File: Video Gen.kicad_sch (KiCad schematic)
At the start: 35 parts, among them J18 Aux Video, K14 RCA Connector, Q3 2N3904

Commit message: more tracing
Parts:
- K14: DigiKey (none) -> PJRAN1X1U03X-ND
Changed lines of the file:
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@@
       (effects (font (size 1.27 1.27)) hide)
     )
-    (pin "8")
-    (pin "9")
     (pin "1")
     (pin "10")
@@
     (pin "6")
     (pin "7")
+    (pin "8")
+    (pin "9")
     (instances
       (project "AppleII"
@@
     (pin "1")
     (pin "2")
-    (pin "4")
-    (pin "7")
-    (pin "8")
-    (pin "3")
-    (pin "6")
+    (pin "3")
+    (pin "4")
+    (pin "6")
+    (pin "7")
+    (pin "8")
     (instances
       (project "AppleII"
@@
       (effects (font (size 1.27 1.27)) hide)
     )
+    (pin "1")
+    (pin "2")
+    (pin "3")
+    (pin "4")
+    (pin "5")
+    (pin "6")
     (pin "8")
     (pin "9")
+    (pin "10")
     (pin "11")
-    (pin "7")
-    (pin "6")
-    (pin "10")
+    (pin "12")
+    (pin "13")
     (pin "14")
-    (pin "13")
-    (pin "1")
-    (pin "4")
-    (pin "5")
-    (pin "2")
-    (pin "3")
-    (pin "12")
+    (pin "7")
     (instances
       (project "AppleII"
@@
       (effects (font (size 1.27 1.27)) hide)
     )
-    (property "Datasheet" "" (at 215.392 67.31 0)
-      (effects (font (size 1.27 1.27)) hide)
-    )
+    (property "Datasheet" "https://www.switchcraft.com/assets/1/24/pjran1x1u__x_series_cd.pdf?4664" (at 215.392 67.31 0)
+      (effects (font (size 1.27 1.27)) hide)
+    )
+    (property "DigiKey" "PJRAN1X1U03X-ND" (at 215.392 67.31 0)
+      (effects (font (size 1.27 1.27)) hide)
+    )

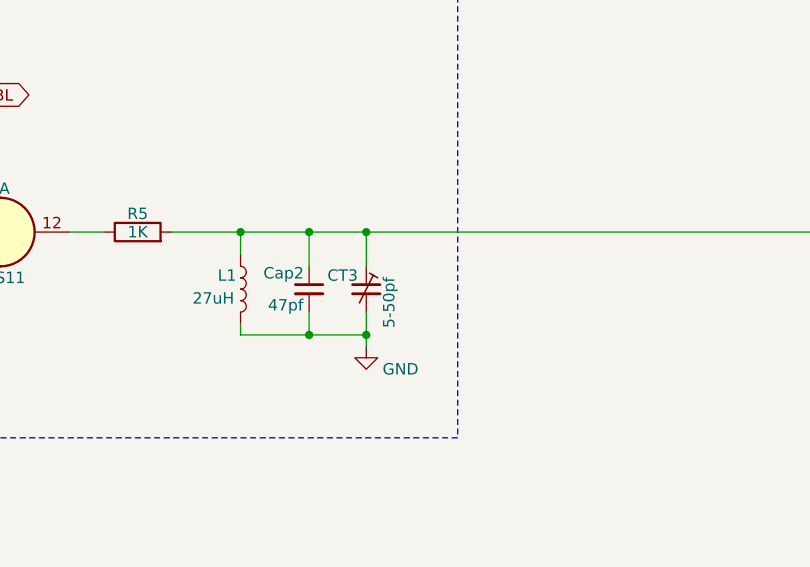
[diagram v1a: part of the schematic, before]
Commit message: more tracing
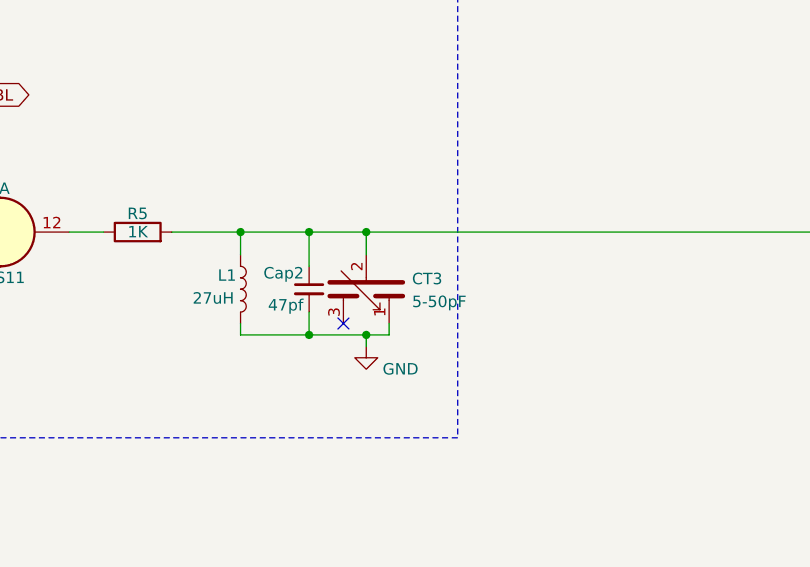
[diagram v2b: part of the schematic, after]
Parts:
- removed CT3: 5-50pf, symbol AppleII-rescue:CTRIM_Small-Device
- added CT3: 5-50pF, Apple-II:COLOUR_TRIM, symbol Device:C_Trim_Differential
- J18: footprint (none) -> Connector_PinHeader_2.54mm:PinHeader_1x04_P2.54mm_Vertical
- Q3: footprint digikey-footprints:TO-92-3 -> Package_TO_SOT_THT:TO-92
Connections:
- net GND: now also CT3.1
- net at Cap2.1, L1.1, R5.2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: now also CT3.2
- no-connect marks 7 -> 8
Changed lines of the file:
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@@
   (no_connect (at 425.45 309.88))
   (no_connect (at 425.45 304.8))
+  (no_connect (at 119.38 201.93))
   (no_connect (at 425.45 240.03))
   (no_connect (at 485.14 170.18))
@@
     (stroke (width 0) (type default))
   )
-  (wire (pts (xy 121.92 200.66) (xy 121.92 203.2))
+  (wire (pts (xy 124.46 201.93) (xy 124.46 203.2))
     (stroke (width 0) (type default))
   )
@@
     (stroke (width 0) (type default))
   )
+  (wire (pts (xy 124.46 203.2) (xy 121.92 203.2))
+    (stroke (width 0) (type default))
+  )
   (wire (pts (xy 196.85 71.12) (xy 205.74 71.12))
     (stroke (width 0) (type default))
@@
     (stroke (width 0) (type default))
   )
-  (wire (pts (xy 121.92 195.58) (xy 121.92 191.77))
+  (wire (pts (xy 121.92 194.31) (xy 121.92 191.77))
     (stroke (width 0) (type default))
   )
@@
     )
   )
-  (symbol (lib_id "AppleII-rescue:CTRIM_Small-Device") (at 121.92 198.12 0) (unit 1)
-    (in_bom yes) (on_board yes) (dnp no)
-    (property "Reference" "CT3" (at 117.602 196.596 0)
-      (effects (font (size 1.27 1.27)) (justify left))
-    )
-    (property "Value" "5-50pf" (at 124.46 202.438 90)
-      (effects (font (size 1.27 1.27)) (justify left))
-    )
-    (property "Footprint" "" (at 121.92 198.12 0)
-      (effects (font (size 1.27 1.27)) hide)
-    )
-    (property "Datasheet" "~" (at 121.92 198.12 0)
-      (effects (font (size 1.27 1.27)) hide)
-    )
-    (pin "1")
-    (pin "2")
-    (instances
-      (project "AppleII"
-        (path "/f1f08369-4db3-46f7-9b89-a5d3cfbed55a/00000000-0000-0000-0000-0000632bf564"
-          (reference "CT3") (unit 1)
-        )
-      )
-    )
-  )
   (symbol (lib_id "power:GND") (at 121.92 204.47 0) (unit 1)
     (in_bom yes) (on_board yes) (dnp no)
@@
       (effects (font (size 1.27 1.27)) (justify right))
     )
-    (property "Footprint" "" (at 172.72 59.69 0)
+    (property "Footprint" "Connector_PinHeader_2.54mm:PinHeader_1x04_P2.54mm_Vertical" (at 172.72 59.69 0)
       (effects (font (size 1.27 1.27)) hide)
     )
@@
       (effects (font (size 1.524 1.524)) (justify left))
     )
-    (property "Footprint" "digikey-footprints:TO-92-3" (at 168.91 92.71 0)
+    (property "Footprint" "Package_TO_SOT_THT:TO-92" (at 168.91 92.71 0)
       (effects (font (size 1.524 1.524)) (justify left) hide)
     )
@@
         )
       )
+    )
+  )
+  (symbol (lib_id "Device:C_Trim_Differential") (at 121.92 198.12 180) (unit 1)
+    (in_bom yes) (on_board yes) (dnp no) (fields_autoplaced)
+    (property "Reference" "CT3" (at 127 196.977 0)
+      (effects (font (size 1.27 1.27)) (justify right))
+    )
+    (property "Value" "5-50pF" (at 127 199.517 0)
+      (effects (font (size 1.27 1.27)) (justify right))
+    )
+    (property "Footprint" "Apple-II:COLOUR_TRIM" (at 121.92 198.12 0)
+      (effects (font (size 1.27 1.27)) hide)
+    )
+    (property "Datasheet" "https://www.vishay.com/docs/28528/bfc2808-10mm.pdf" (at 121.92 198.12 0)
+      (effects (font (size 1.27 1.27)) hide)
+    )
+    (property "DigiKey" "BFC280831659-ND" (at 121.92 198.12 0)
+      (effects (font (size 1.27 1.27)) hide)
+    )
+    (pin "1")
+    (pin "2")
+    (pin "3")
+    (instances
+      (project "AppleII"
+        (path "/f1f08369-4db3-46f7-9b89-a5d3cfbed55a/00000000-0000-0000-0000-0000632bf564"
+          (reference "CT3") (unit 1)
+        )
+      )

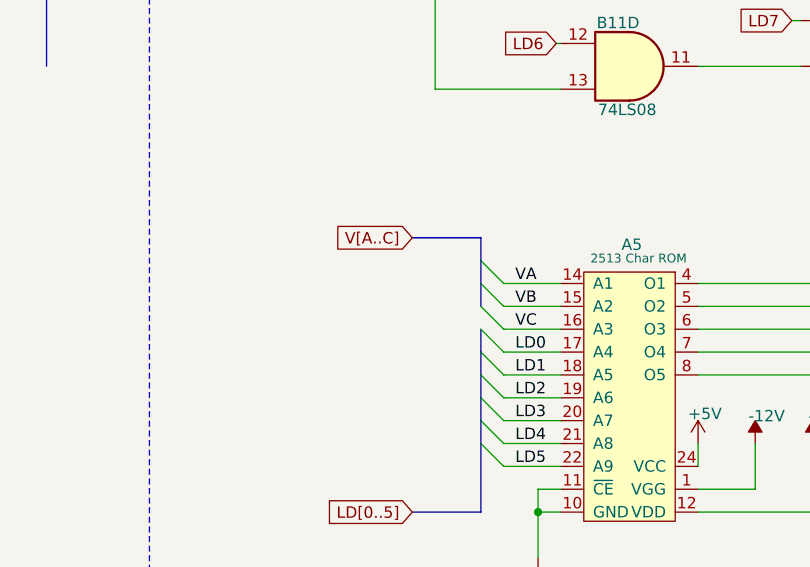
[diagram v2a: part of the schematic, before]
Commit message: more tracing
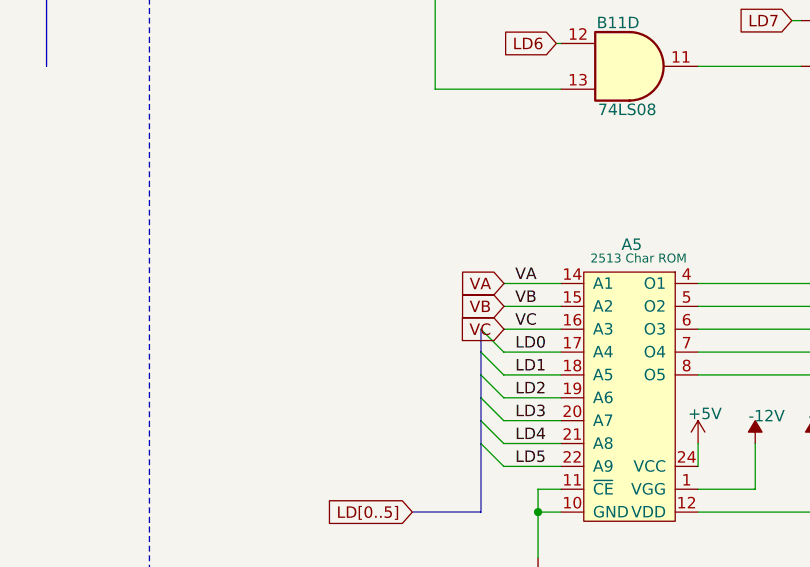
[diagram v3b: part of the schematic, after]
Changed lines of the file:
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@@
-    (stroke (width 0) (type default))
-  )
-  (bus_entry (at 302.26 135.89) (size 2.54 2.54)
     (stroke (width 0) (type default))
   )
@@
     (stroke (width 0) (type default))
   )
-  (bus_entry (at 302.26 138.43) (size 2.54 2.54)
-    (stroke (width 0) (type default))
-  )
   (bus_entry (at 395.224 242.57) (size 2.54 2.54)
     (stroke (width 0) (type default))
   )
-  (bus_entry (at 302.26 133.35) (size 2.54 2.54)
-    (stroke (width 0) (type default))
-  )
   (bus_entry (at 395.224 234.95) (size 2.54 2.54)
     (stroke (width 0) (type default))
@@
     (stroke (width 0) (type default))
   )
-  (bus (pts (xy 294.64 130.81) (xy 302.26 130.81))
-    (stroke (width 0) (type default))
-  )
   (wire (pts (xy 36.83 374.65) (xy 34.29 374.65))
     (stroke (width 0) (type default))
@@
     (stroke (width 0) (type default))
   )
-  (bus (pts (xy 302.26 133.35) (xy 302.26 130.81))
-    (stroke (width 0) (type default))
-  )
   (wire (pts (xy 153.67 95.25) (xy 157.48 95.25))
     (stroke (width 0) (type default))
@@
     (stroke (width 0) (type default))
   )
-  (bus (pts (xy 302.26 138.43) (xy 302.26 135.89))
-    (stroke (width 0) (type default))
-  )
   (wire (pts (xy 149.86 63.5) (xy 149.86 64.77))
     (stroke (width 0) (type default))
@@
   )
   (wire (pts (xy 304.8 146.05) (xy 311.15 146.05))
-    (stroke (width 0) (type default))
-  )
-  (bus (pts (xy 302.26 135.89) (xy 302.26 133.35))
     (stroke (width 0) (type default))
   )
@@
     )
   )
+  (global_label "VB" (shape input) (at 304.8227 138.43 180) (fields_autoplaced)
+    (effects (font (size 1.27 1.27)) (justify right))
+    (property "Intersheetrefs" "${INTERSHEET_REFS}" (at 300.1331 138.43 0)
+      (effects (font (size 1.27 1.27)) (justify right) hide)
+    )
+  )
   (global_label "HIRES" (shape output) (at 151.13 325.12 0)
     (effects (font (size 1.27 1.27)) (justify left))
@@
     )
   )
+  (global_label "VA" (shape input) (at 304.8227 135.89 180) (fields_autoplaced)
+    (effects (font (size 1.27 1.27)) (justify right))
+    (property "Intersheetrefs" "${INTERSHEET_REFS}" (at 300.3145 135.89 0)
+      (effects (font (size 1.27 1.27)) (justify right) hide)
+    )
+  )
   (global_label "V2" (shape input) (at 43.942 322.58 180)
     (effects (font (size 1.27 1.27)) (justify right))
@@
     )
   )
-  (global_label "V[A..C]" (shape input) (at 294.64 130.81 180)
-    (effects (font (size 1.27 1.27)) (justify right))
-    (property "Intersheetrefs" "${INTERSHEET_REFS}" (at 294.64 130.81 0)
-      (effects (font (size 1.27 1.27)) hide)
-    )
-  )
   (global_label "LD[0..7]" (shape input) (at 395.224 232.918 0)
     (effects (font (size 1.27 1.27)) (justify left))
@@
     )
   )
+  (global_label "VC" (shape input) (at 304.8227 140.97 180) (fields_autoplaced)
+    (effects (font (size 1.27 1.27)) (justify right))
+    (property "Intersheetrefs" "${INTERSHEET_REFS}" (at 300.1331 140.97 0)
+      (effects (font (size 1.27 1.27)) (justify right) hide)
+    )
+  )
